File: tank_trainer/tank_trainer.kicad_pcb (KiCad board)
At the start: 2 copper layers, 33 x 52 mm, 20 parts, among them U1 L7805, U2 ATMEGA328P-PU, Y1 Crystal

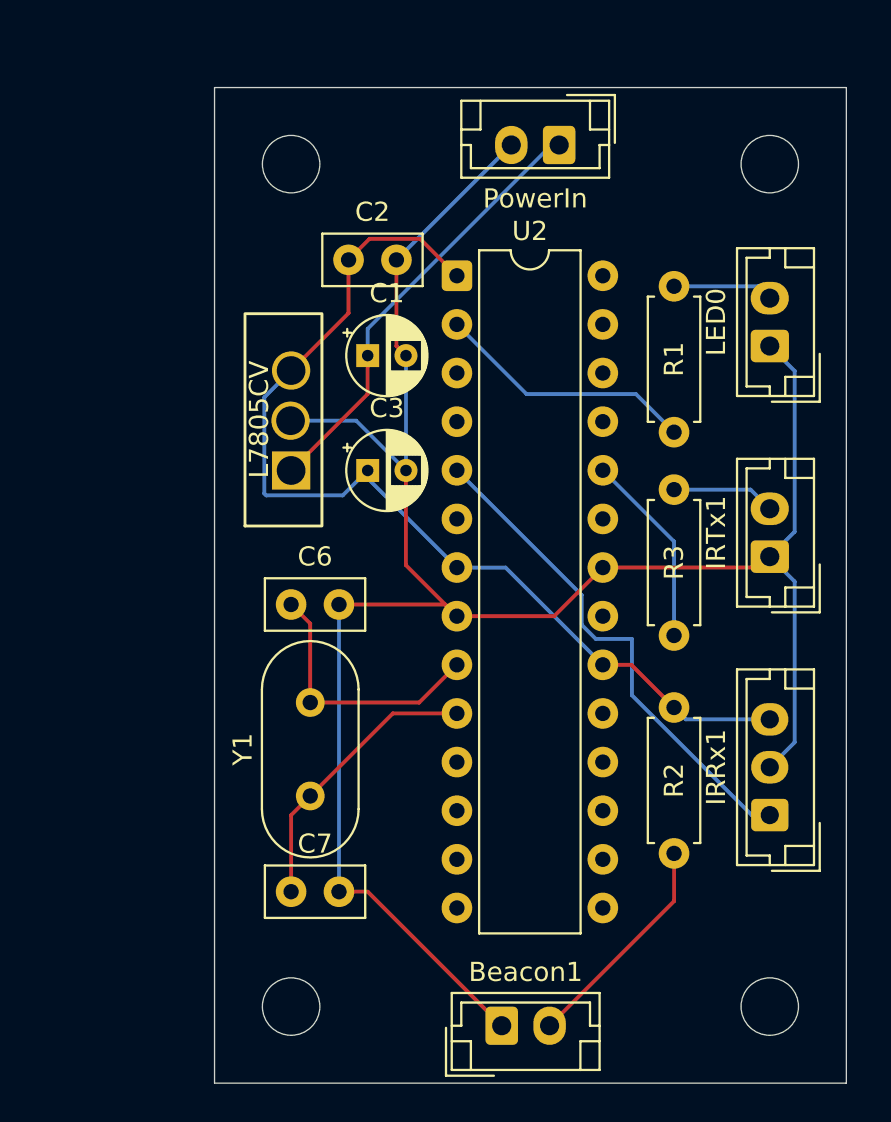
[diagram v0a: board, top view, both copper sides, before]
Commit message: update tank trainer to add programming header
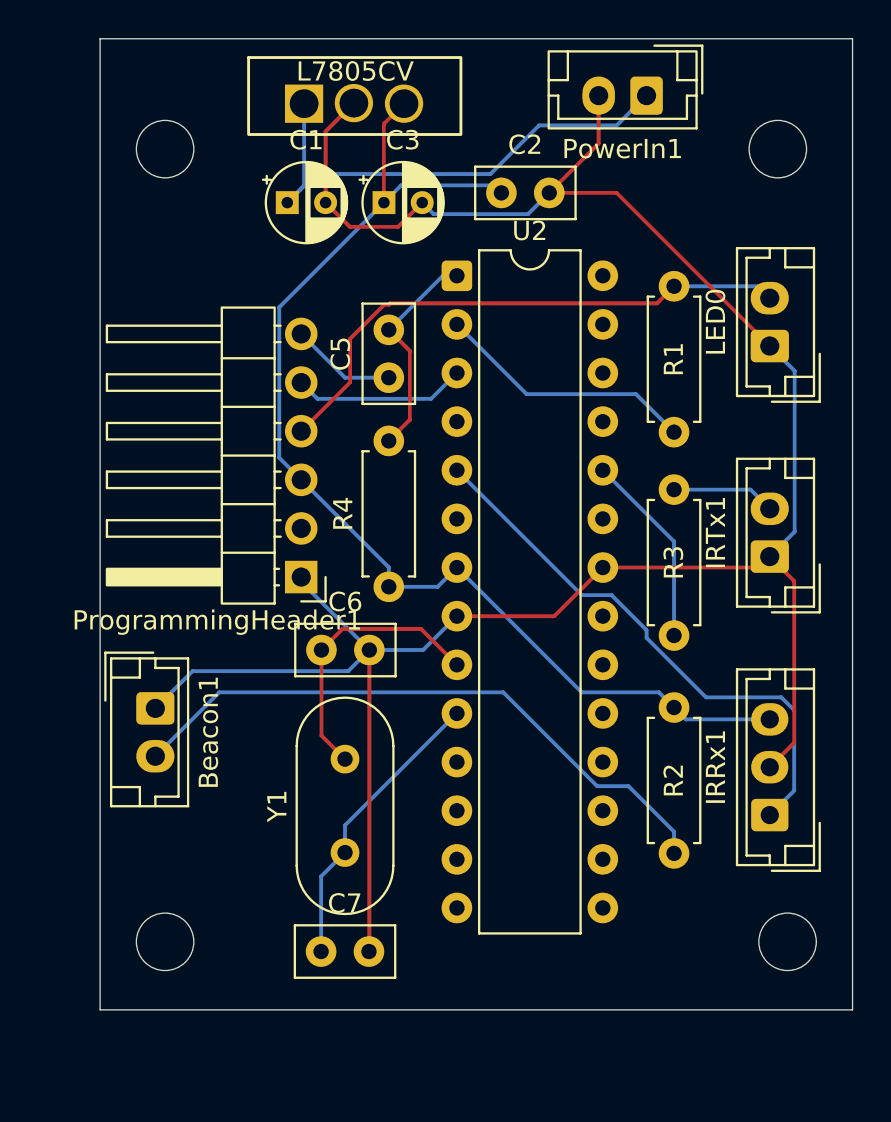
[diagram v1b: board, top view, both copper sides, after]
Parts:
- removed PowerIn: PowerIn, Connector_JST:JST_EH_B2B-EH-A_1x02_P2.50mm_Vertical
- added C5: 100nF, Capacitor_THT:C_Disc_D5.0mm_W2.5mm_P2.50mm, F.Cu at (54.1, 89.2)
- added PowerIn1: PowerIn, Connector_JST:JST_EH_B2B-EH-A_1x02_P2.50mm_Vertical, F.Cu at (67.6, 74.4)
- added ProgrammingHeader1: Programming Header, Connector_PinHeader_2.54mm:PinHeader_1x06_P2.54mm_Horizontal, F.Cu at (49.5, 99.6)
- added R4: R, Resistor_THT:R_Axial_DIN0207_L6.3mm_D2.5mm_P7.62mm_Horizontal, F.Cu at (54.1, 100.1)
- moved Beacon1 24.5 mm to (41.9, 106.4), turned to -90 degrees
- moved U1 21.1 mm to (48.7, 73.9), turned to 0 degrees
- moved C3 14.0 mm to (53.8, 80.0)
- moved C1 9.03 mm to (48.8, 80.0)
- moved C2 8.72 mm to (60.0, 79.5)
- moved H4 7.40 mm to (42.4, 118.6)
- moved H1 6.63 mm to (42.4, 77.2)
- moved H5 3.51 mm to (74.9, 118.6)
- moved C7 3.50 mm to (50.6, 119.1)
- moved Y1 3.47 mm to (51.8, 114.0)
- moved C6 2.86 mm to (50.6, 103.4)
- moved H3 0.89 mm to (74.4, 77.2)
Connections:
- net 9V renamed Net-(PowerIn1-Pin_1)
- net Net-(LED0-Pin_2) renamed Rx
- U2 pad 1: 4.5V -> Net-(U2-(PCINT14/~{RESET})PC6)
- U2 pad 20: 4.5V -> unconnected-(U2-AVCC-Pad20)
- U2 pad 3: unconnected-(U2-(PCINT17/TXD)PD1-Pad3) -> Tx
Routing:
- net Rx: track 5.26 -> 29.2 mm
- net Net-(Beacon1-Pin_2): track 11.7 -> 32.6 mm
- net Net-(U2-(PCINT14/~{RESET})PC6): track 0.00 -> 11.4 mm
- net GND: track 110.1 -> 120.8 mm
- net Tx: track 0.00 -> 9.04 mm
- net 4.5V: track 53.9 -> 60.6 mm
- net Net-(ProgrammingHeader1-Pin_6): track 0.00 -> 5.52 mm
- net Net-(PowerIn1-Pin_1): track 23.0 -> 26.6 mm
- net Net-(IRRx1-Pin_1): track 26.4 -> 29.0 mm
- net Net-(U2-(PCINT7/XTAL2/TOSC2)PB7): track 14.9 -> 15.4 mm
- net Net-(U2-(PCINT6/XTAL1/TOSC1)PB6): track 14.0 -> 14.5 mm
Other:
- board size 33 x 52 mm -> 39.3 x 50.7 mm

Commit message: tank trainer v0.2 (whoops ... forgot the button)
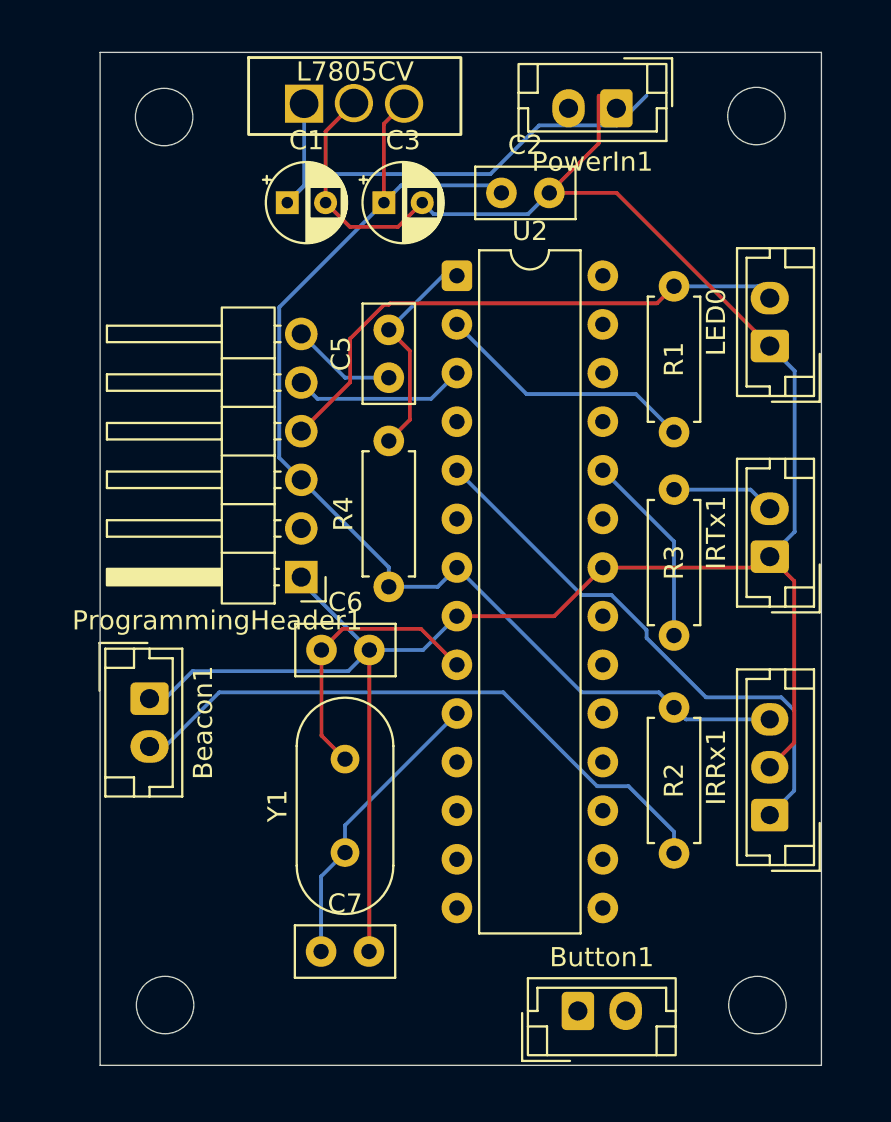
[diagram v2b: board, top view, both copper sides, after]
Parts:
- added Button1: Conn_01x02_Pin, Connector_JST:JST_EH_B2B-EH-A_1x02_P2.50mm_Vertical, F.Cu at (64.0, 122.2)
- moved H5 3.66 mm to (73.4, 121.9)
- moved H4 3.30 mm to (42.4, 121.9)
- moved H3 2.06 mm to (73.3, 75.5)
- moved PowerIn1 1.71 mm to (66.0, 75.1)
- moved H1 1.68 mm to (42.4, 75.5)
- moved Beacon1 0.59 mm to (41.6, 105.9)
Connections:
- U2 pad 4: unconnected-(U2-(PCINT18/INT0)PD2-Pad4) -> Net-(Button1-Pin_2)
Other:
- board size 39.3 x 50.7 mm -> 37.7 x 52.9 mm
- board text added: "Laser Tag Robot Tank Tank Trainer v0.2"
- board text removed: "Laser Tag Robot Tank Tank Trainer v0.1"
